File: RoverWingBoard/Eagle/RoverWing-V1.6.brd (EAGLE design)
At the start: 81.3 x 81.3 mm, 89 parts, among them J1 XT30UPB-M, J10 HEADER-PH-4P, J11 HEADER-PH-3P, J12 HEADER-3X04, J13 HEADER-3X06", J14 HEADER-2X16, J15 HEADER-2X12, J16 DF13-4P-1.25DSA, J17 DF13-6P-1.25DSA, J2 HEADER-VH, J3 HEADER-VH, J4 HEADER-PH-4P, J5 HEADER-PH-4P, J6 BM04B-SRSS-TB(LF)(SN), J8 HEADER-PH-4P, J9 HEADER-PH-4P, SW1 SW-TACTILE-4.5X4.5_SMD, U1 ATSAMD21G, U2 MP2225, U3 PMIC-AZ1117EH-3.3, U5 DRV8871, U6 DRV8871, U7 74AHCT1G125DBV, U9 ICM-42605

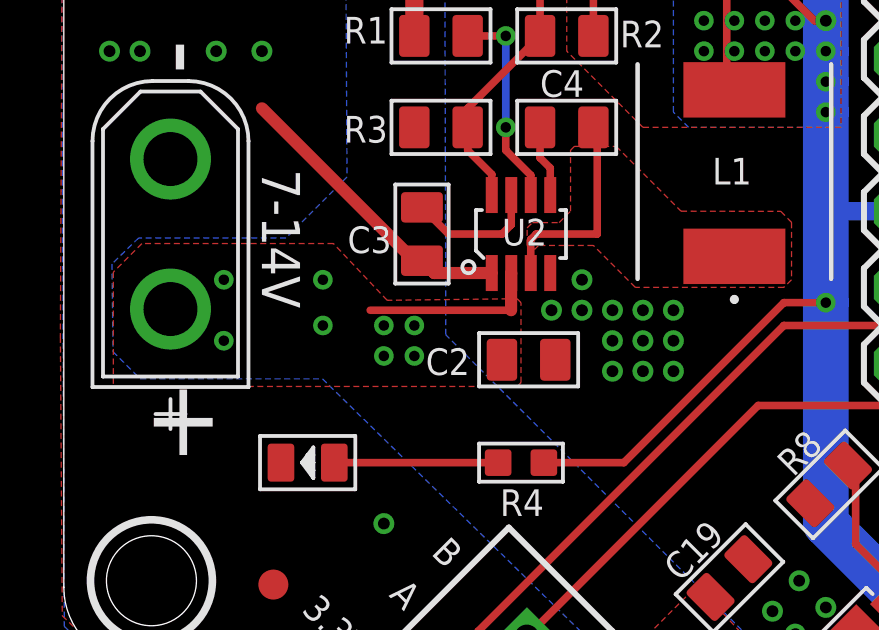
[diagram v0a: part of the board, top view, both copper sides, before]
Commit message: docs update
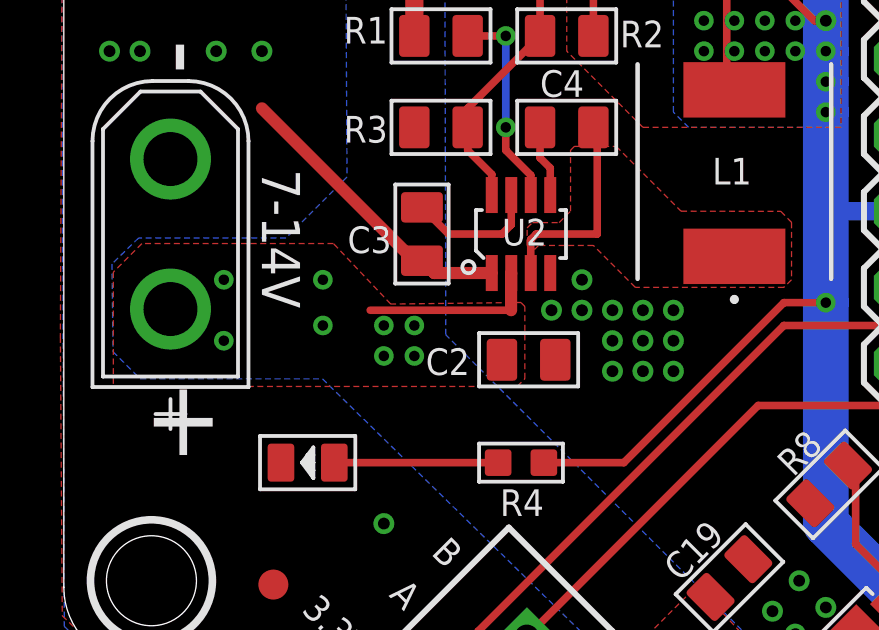
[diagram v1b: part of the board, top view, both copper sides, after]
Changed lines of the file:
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@@
 <via x="-28.956" y="4.572" extent="1-16" drill="0.35"/>
 <polygon width="0.0254" layer="1" thermals="no">
-<vertex x="-25.4" y="-6.858"/>
-<vertex x="-25.530075" y="-6.727925"/>
-<vertex x="-29.8613125" y="-6.781003125"/>
+<vertex x="-25.273" y="-6.985"/>
+<vertex x="-25.4046125" y="-6.8533875"/>
+<vertex x="-29.74246875" y="-6.906546875"/>
 <vertex x="-31.651875" y="-4.8895"/>
 <vertex x="-38.0365" y="-4.8895"/>
@@
 <vertex x="-38.989" y="-9.652"/>
 <vertex x="-25.527" y="-9.652"/>
-<vertex x="-25.4" y="-9.525"/>
+<vertex x="-25.273" y="-9.398"/>
 </polygon>
 <via x="-29.972" y="-7.62" extent="1-16" drill="0.35"/>
